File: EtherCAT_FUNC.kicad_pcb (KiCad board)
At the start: 2 copper layers, 33.7 x 62.4 mm, 58 parts, among them J1 axt430124, J10 Conn_01x02, J11 Conn_01x02, J12 Conn_01x02, J13 Conn_01x02, J14 Conn_01x02, J15 Conn_01x02, J16 Conn_01x02, J2 Conn_01x02, J3 Conn_01x02, J4 Conn_01x04, J5 Conn_01x02, J6 Conn_01x04, J7 Conn_01x04, J8 Conn_01x03, J9 Conn_01x02, U1 SY8303AAIC, U2 TJA1051T-3, U3 TJA1051T-3, U6 ESDS314

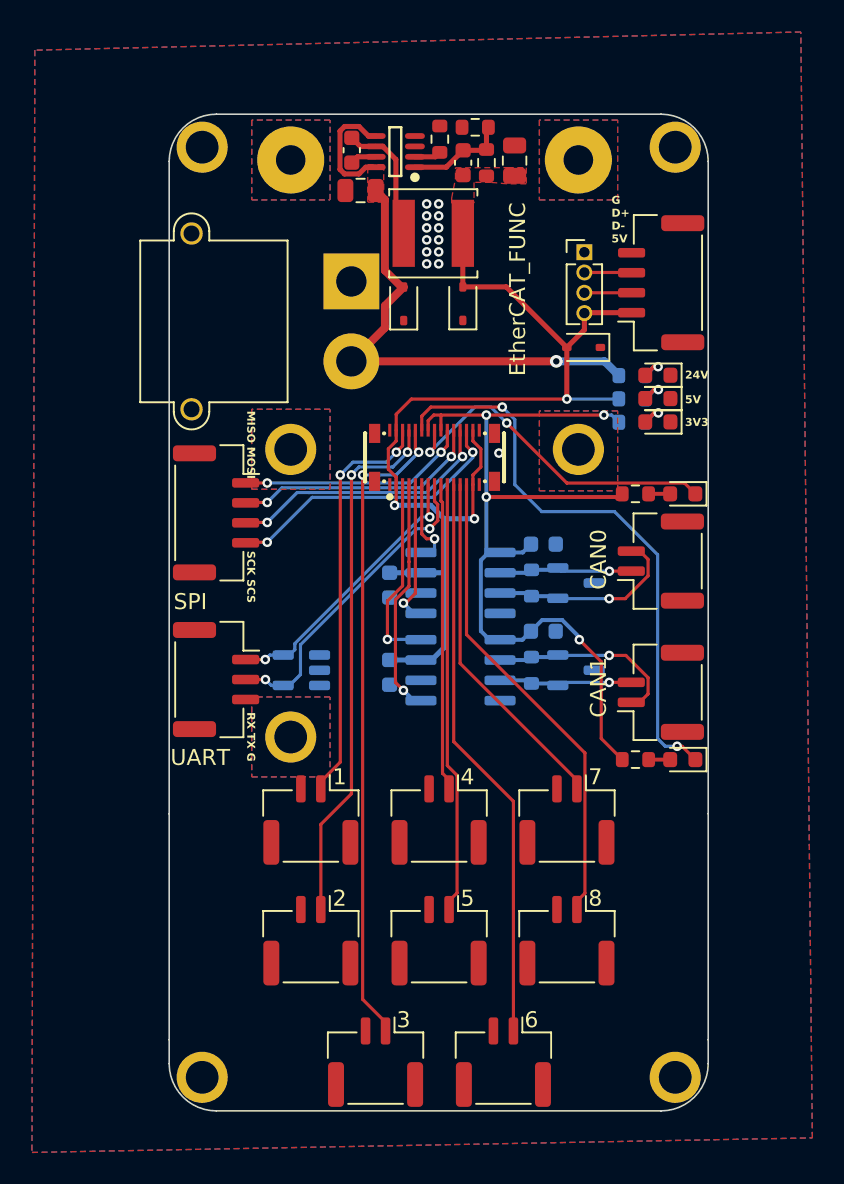
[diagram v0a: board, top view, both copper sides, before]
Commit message: Official version
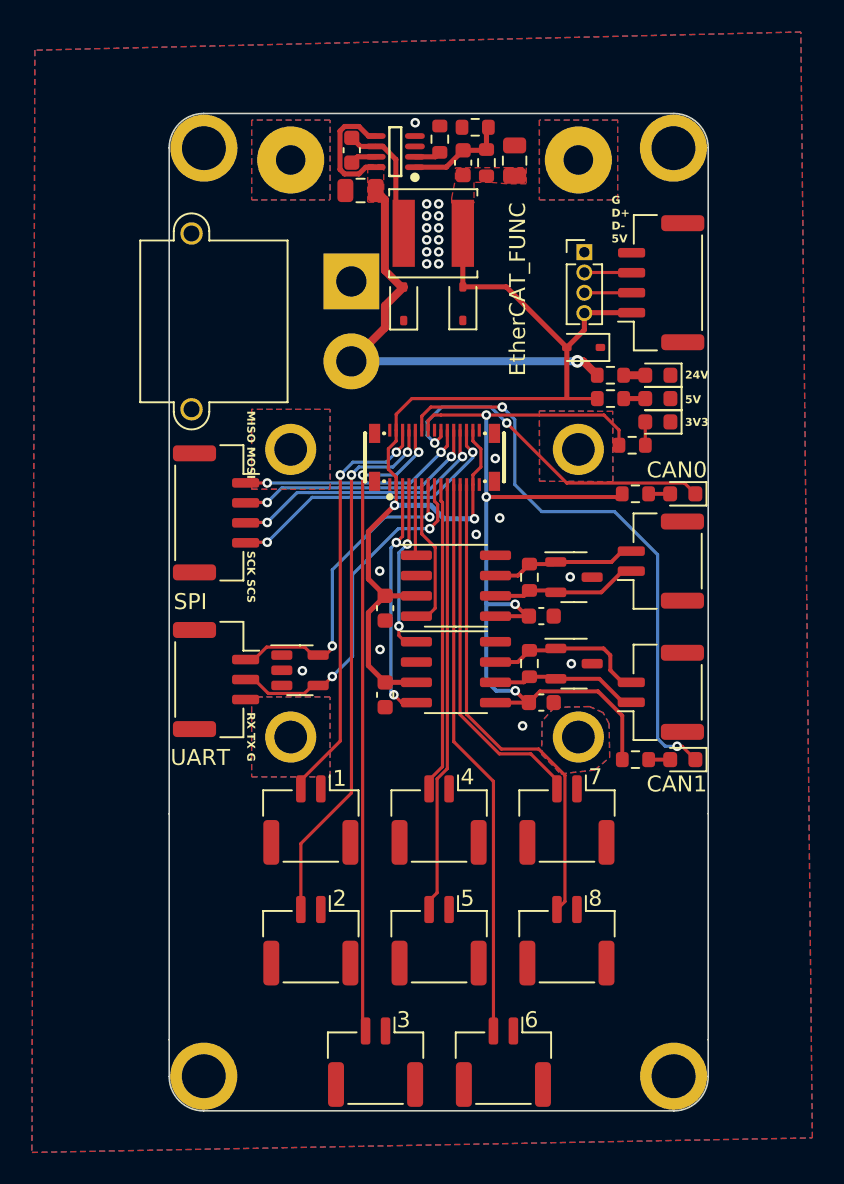
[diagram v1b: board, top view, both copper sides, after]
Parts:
- added H10: MountingHole, EXTRA IC:M1.6, F.Cu at (162.7, 109.1)
- C5, C6, C7, C8, R10, R6, R7, R8, R9, U2, U3, U4, U5, U6: moved to F.Cu
- H4, H5, H6, H7: footprint EXTRA IC:M1.6 -> EXTRA IC:M2_HOLE
- H8, H9: footprint EXTRA IC:M2 -> EXTRA IC:M2_noHOLE
- moved C6 4.50 mm to (160.4, 101.5)
- moved C5 4.46 mm to (160.4, 107.0)
- moved C8 1.47 mm to (150.7, 101.0)
- moved R8 1.44 mm to (166.1, 90.8)
- moved C7 1.43 mm to (150.7, 106.5)
- moved R10 1.35 mm to (164.7, 86.5)
- moved R9 1.35 mm to (164.8, 87.9)
- moved R7 0.44 mm to (159.7, 104.5), turned to -90 degrees
- moved U5 0.43 mm to (162.5, 104.5)
- moved U4 0.39 mm to (162.5, 99.1)
- moved R6 0.38 mm to (159.7, 99.1), turned to -90 degrees
- moved U2 0.33 mm to (155.1, 99.6)
- moved U3 0.31 mm to (155.1, 105.0)
- moved H6 0.13 mm to (139.3, 72.3)
- moved H7 0.13 mm to (168.7, 72.3)
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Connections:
- J1 pad 22: 3V3 -> LED_CAN0
- J1 pad 23: LED_CAN0 -> GND
- J10 pad 1: /GPIO2 -> GND
- J10 pad 2: GND -> /GPIO2
- J11 pad 1: /GPIO3 -> GND
- J11 pad 2: GND -> /GPIO3
- J12 pad 1: /GPIO4 -> GND
- J12 pad 2: GND -> /GPIO4
- J13 pad 1: /GPIO5 -> GND
- J13 pad 2: GND -> /GPIO5
- J14 pad 1: /GPIO6 -> GND
- J14 pad 2: GND -> /GPIO6
- J15 pad 1: /GPIO7 -> GND
- J15 pad 2: GND -> /GPIO7
- J16 pad 1: /GPIO8 -> GND
- J16 pad 2: GND -> /GPIO8
- J9 pad 1: /GPIO1 -> GND
- J9 pad 2: GND -> /GPIO1
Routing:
- net 3V3: track 54.8 -> 59.6 mm
- net /CAN/FDCAN1_TX: track 9.17 -> 4.45 mm, vias 1 -> 0
- net /CAN/FDCAN1_RX: track 4.91 -> 9.47 mm, vias 1 -> 0
- net /CAN/FDCAN2_TX: track 14.8 -> 11.0 mm, vias 1 -> 2
- net /CAN/CAN0_H: track 12.3 -> 9.13 mm, vias 1 -> 0
- net /UART_RX: track 17.5 -> 20.6 mm
- net /CAN/CAN1_L: track 12.3 -> 9.30 mm, vias 1 -> 0
- net /CAN/FDCAN2_RX: track 12.2 -> 15.1 mm, vias 1 -> 2
- net /UART_TX: track 19.9 -> 22.2 mm
- net /CAN/CAN1_H: track 8.42 -> 10.3 mm, vias 1 -> 0
- net +24V: track 37.5 -> 36.1 mm
- net /GPIO8: track 29.9 -> 30.7 mm
- net /CAN/CAN0_L: track 8.42 -> 9.24 mm, vias 1 -> 0
- net Net-(D4-A): track 2.12 -> 1.35 mm, vias 1 -> 0
- net Net-(D5-A): track 2.07 -> 1.36 mm, vias 1 -> 0
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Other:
- outline, holes or cut-outs redrawn
